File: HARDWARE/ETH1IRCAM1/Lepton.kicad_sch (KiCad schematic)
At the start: 14 parts, among them Q501 MMBT3904, U501 105028-1001 + Lepton 3.1R, X501 ASEMB-25.000MHZ-LY-T

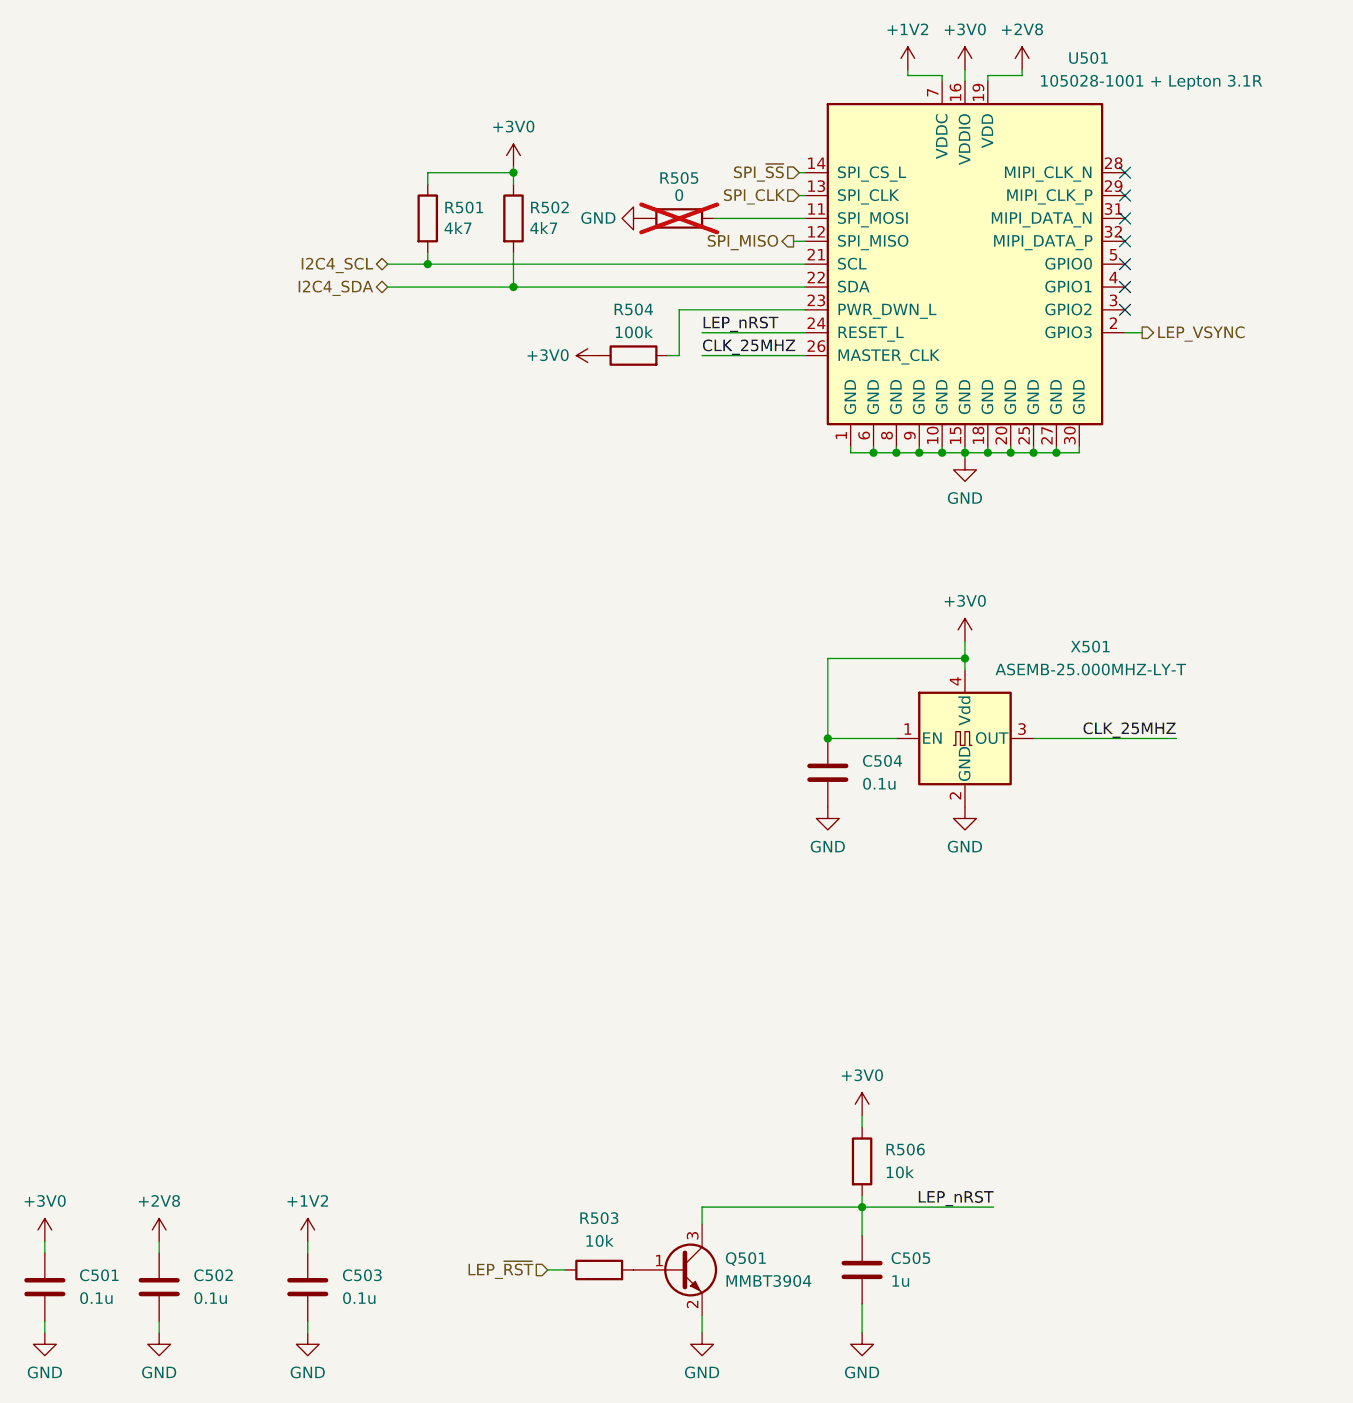
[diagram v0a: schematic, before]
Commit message: Bug fixes
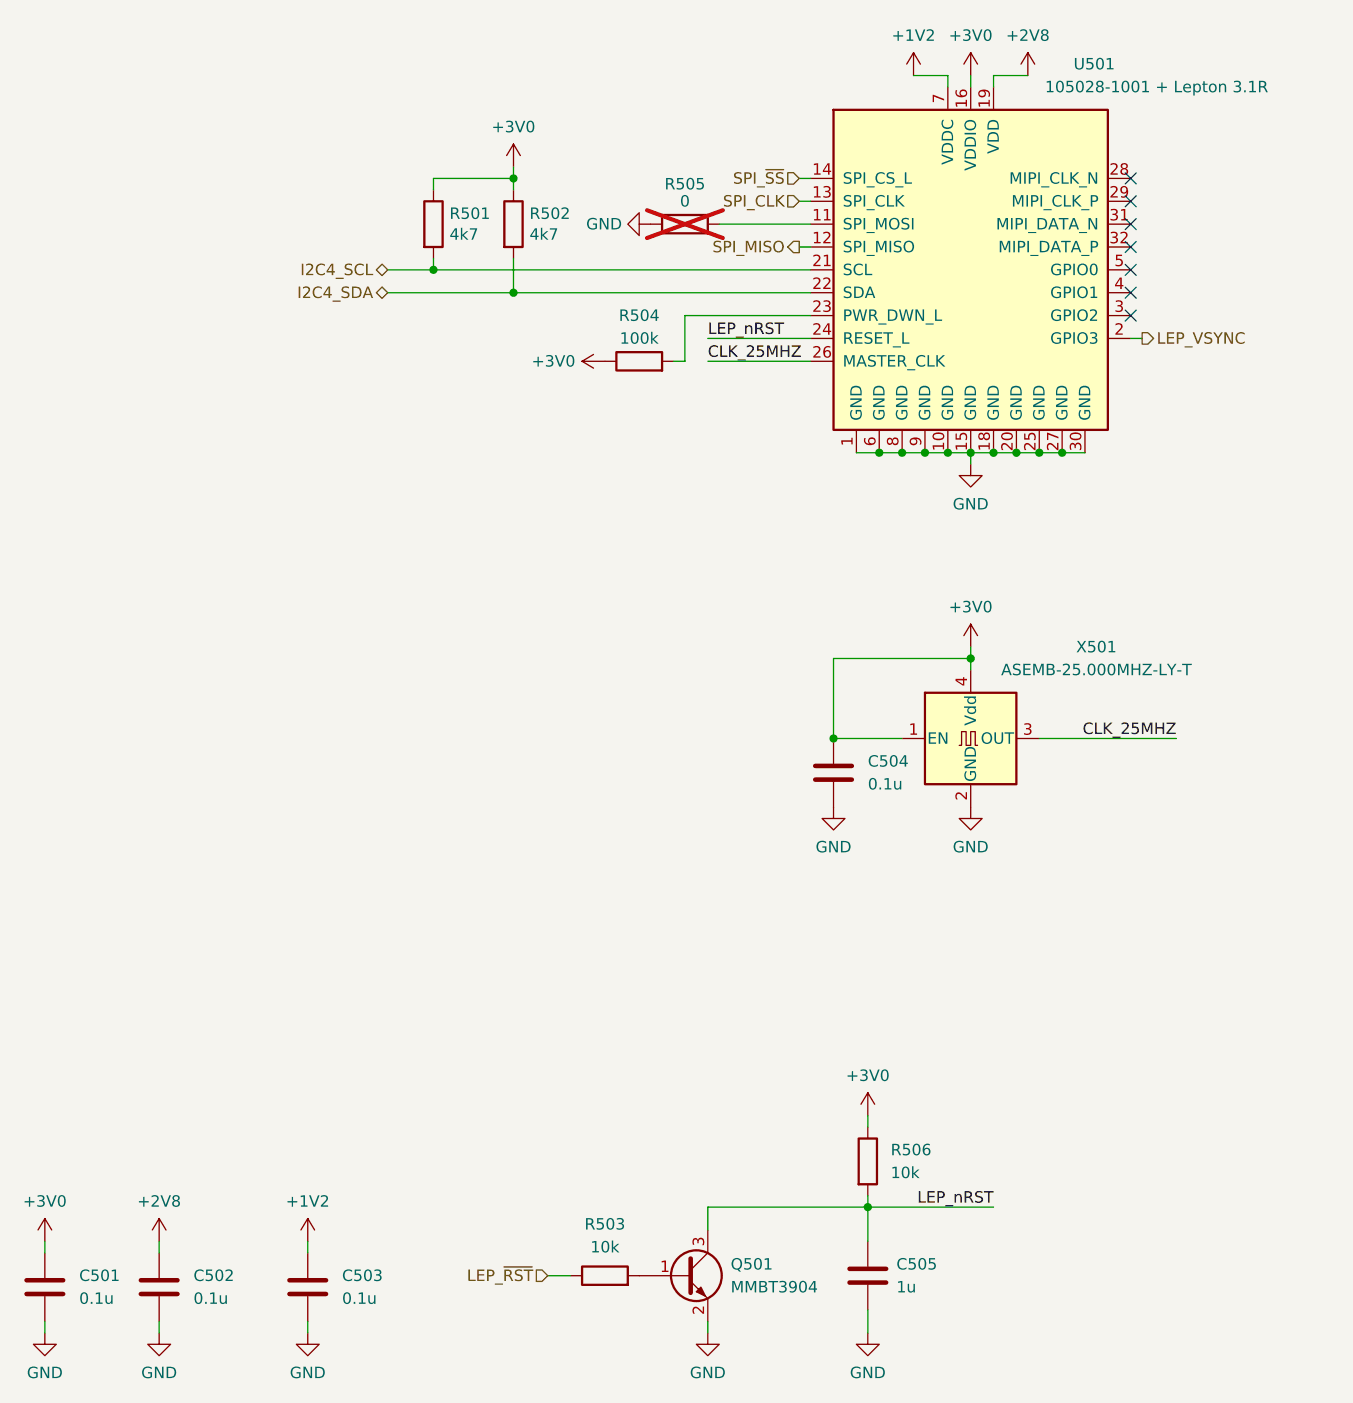
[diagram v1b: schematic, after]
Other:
- moved on the sheet: C504, C505, Q501, R501, R502, R503, R504, R505, R506, U501, X501
